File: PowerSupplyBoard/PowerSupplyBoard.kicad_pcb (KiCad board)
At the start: 4 copper layers, 50 x 75 mm, 80 parts, among them J101 BATTERY, J102 DATA2, J103 USB_C, J104 PWR, J105 DATA1, J106 USB_B_Micro, Q101 BSH205G2A, Q102 TD6790, Q103 TD6790, Q104 TD6790, SW101 SW_SPDT, U101 TPS63021, U102 MCP73834T, U103 TC7662Bx0A, U104 TC7662Bx0A, U105 CS5173

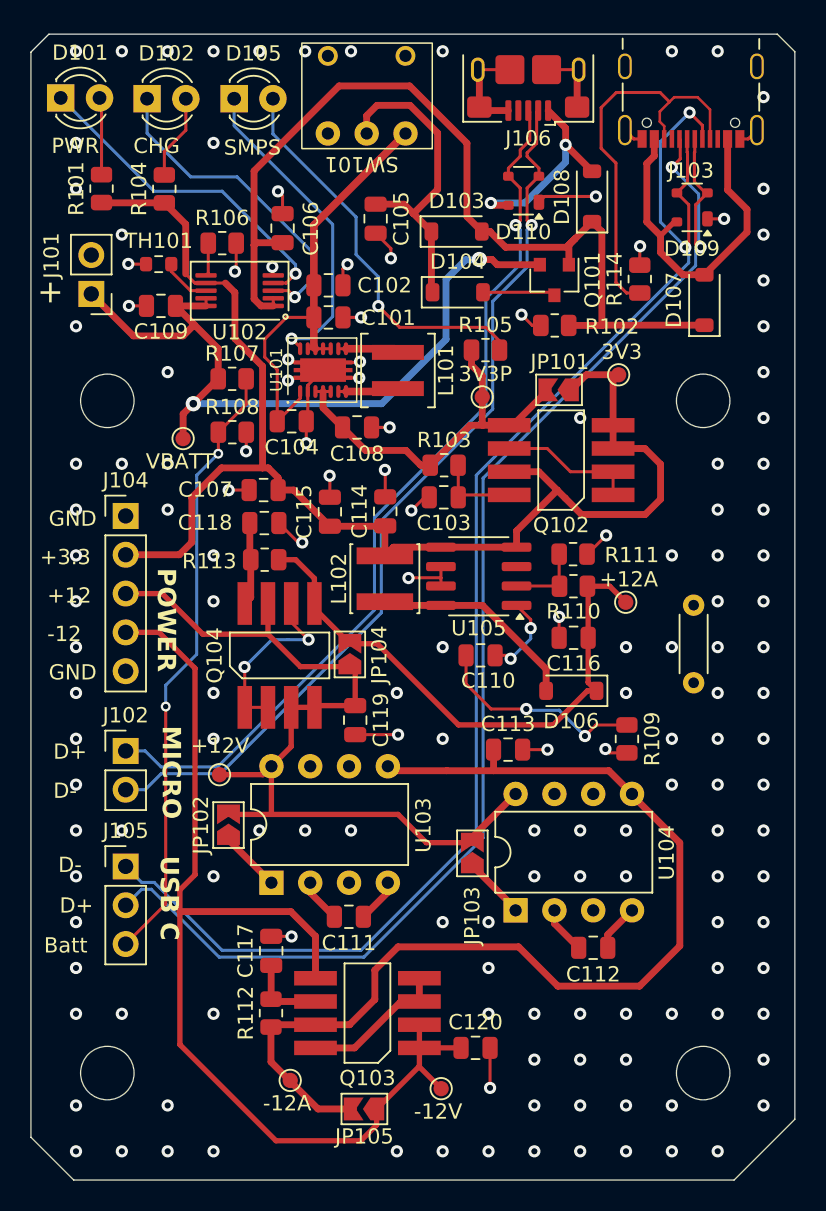
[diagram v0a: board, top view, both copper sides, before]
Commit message: Power board rev 3
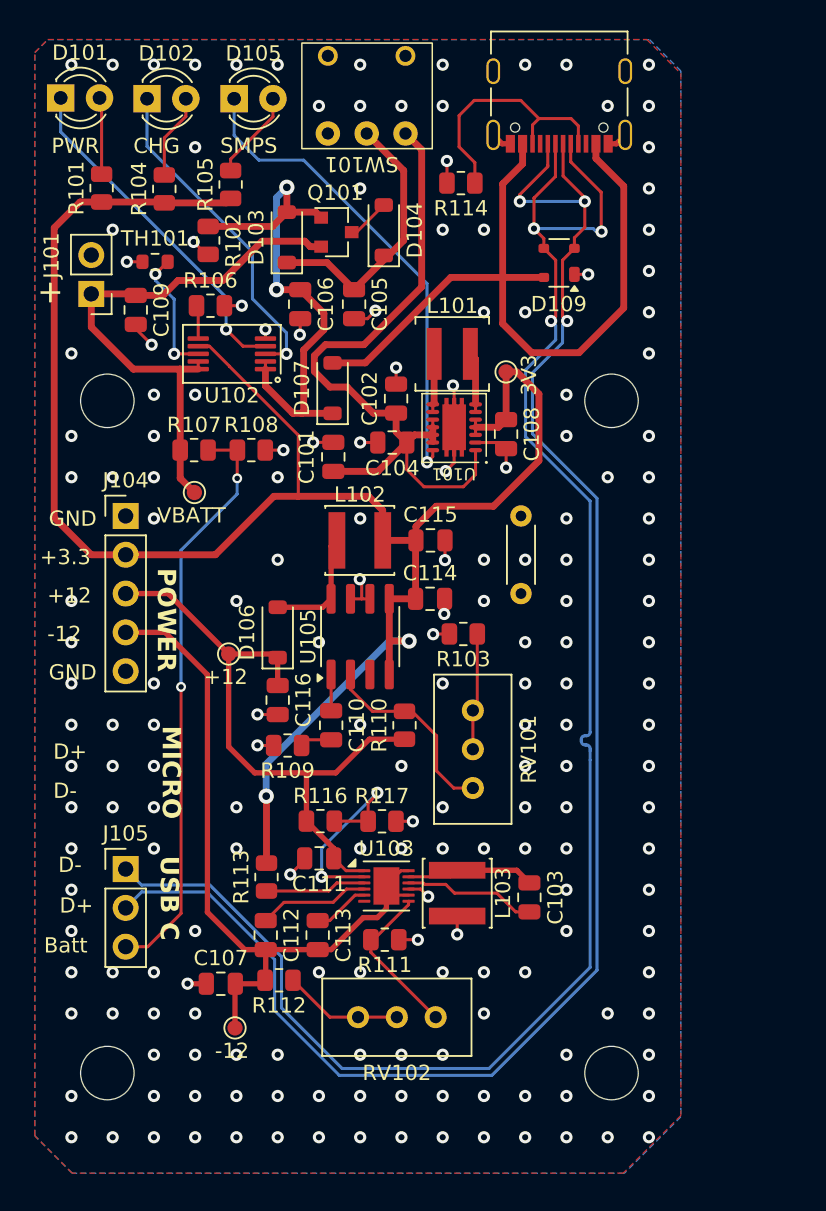
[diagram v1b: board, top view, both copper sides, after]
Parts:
- removed C117, C118: 1u, Capacitor_SMD:C_0805_2012Metric
- removed C119, C120: 100n, Capacitor_SMD:C_0805_2012Metric
- removed D108: PMEG3030, Diode_SMD:D_SOD-123
- removed D110: SP0503BAHT, Package_TO_SOT_SMD:SOT-143
- removed J102: DATA2, Connector_PinHeader_2.54mm:PinHeader_1x02_P2.54mm_Vertical
- removed J106: USB_B_Micro, Connector_USB:USB_Micro-B_Amphenol_10118193-0001LF_Horizontal
- removed JP101: DIG_CM, Jumper:SolderJumper-2_Open_TrianglePad_0805
- removed JP102, JP103: INV_HIFREQ, Jumper:SolderJumper-2_Open_TrianglePad_0805
- removed JP104: POS_CM, Jumper:SolderJumper-2_Open_TrianglePad_0805
- removed JP105: NEG_CM, Jumper:SolderJumper-2_Open_TrianglePad_0805
- removed Q102, Q103, Q104: TD6790, PCM_4ms_Package_SOIC:SM-8
- removed TP104: -12A, TestPoint:TestPoint_Pad_D1.0mm_Value
- removed TP106: -12V, TestPoint:TestPoint_Pad_D1.0mm_Value
- removed TP107: +12V, TestPoint:TestPoint_Pad_D1.0mm_Value
- removed U104: TC7662Bx0A, Package_DIP:DIP-8_W7.62mm
- added L103: 22uH, Inductor_SMD:L_Changjiang_FNR4010S, F.Cu at (27.9, 56.2)
- added R116: 330k, Resistor_SMD:R_0805_2012Metric, F.Cu at (18.9, 51.5)
- added R117: 100k, Resistor_SMD:R_0805_2012Metric, F.Cu at (23.0, 51.5)
- added RV101: 10k, Potentiometer_THT:Potentiometer_Bourns_3296W_Vertical, F.Cu at (28.9, 49.3)
- added RV102: 10k, Potentiometer_THT:Potentiometer_Bourns_3296W_Vertical, F.Cu at (26.5, 64.3)
- C103: value 22u -> 100n
- C107: value 100n -> 22u
- C111: value 10u -> 4u7
- C112: value 10u -> 4n7
- C113: value 10u -> 2u2
- R103: value 10k -> 1k
- R111: value 4k7 -> 470k
- R112: value 12k -> 33k
- R113: value 12k -> 4k7
- TP101: value 3V3 -> -12
- TP102: value 3V3P -> 3V3
- TP105: value +12A -> +12
- U103: value TC7662Bx0A -> MAX17578ATC; footprint Package_DIP:DIP-8_W7.62mm -> Package_DFN_QFN:TDFN-12-1EP_3x3mm_P0.4mm_EP1.7x2.45mm
- moved TP101 49.6 mm to (13.4, 65.0), turned to 180 degrees
- moved C107 32.4 mm to (12.4, 62.2), turned to 0 degrees
- moved R111 28.1 mm to (23.2, 59.3), turned to 180 degrees
- moved C103 26.8 mm to (32.6, 56.5), turned to 90 degrees
- moved TP105 26.2 mm to (12.9, 40.6), turned to 180 degrees
- moved D107 25.0 mm to (19.7, 23.2)
- moved R102 23.4 mm to (11.6, 13.5), turned to -90 degrees
- moved R109 22.2 mm to (16.8, 46.6), turned to 180 degrees
- moved C112 21.5 mm to (15.4, 59.0), turned to -90 degrees
- moved R113 20.8 mm to (15.4, 55.2), turned to 90 degrees
- moved R105 19.9 mm to (13.1, 9.84), turned to 90 degrees
- moved C116 19.8 mm to (16.1, 43.6), turned to -90 degrees
- moved D106 19.6 mm to (16.1, 39.2), turned to 90 degrees
- moved C113 17.4 mm to (18.8, 59.0), turned to -90 degrees
- moved Q101 14.6 mm to (20.0, 13.0), turned to 0 degrees
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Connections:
- C103 pad 1: Net-(Q102A-B1) -> Net-(U103-BST)
- C103 pad 2: GND -> Net-(U103-LX)
- C107 pad 1: +3.3V -> GND
- C107 pad 2: GND -> -12V
- C108 pad 1: +3.3VP -> +3.3V
- C111 pad 1: Net-(U103-CAP+) -> +12V
- C111 pad 2: Net-(U103-CAP-) -> GND
- C112 pad 1: Net-(U104-CAP+) -> Net-(U103-SS)
- C112 pad 2: Net-(U104-CAP-) -> -12V
- C113 pad 1: -12VA -> Net-(U103-VCC)
- C113 pad 2: GND -> -12V
- C116 pad 1: +12VA -> +12V
- D106 pad 1: +12VA -> +12V
- R103 pad 1: +3.3VP -> Net-(R103-Pad1)
- R103 pad 2: Net-(Q102A-B1) -> GND
- R105 pad 1: +3.3VP -> +3.3V
- R110 pad 1: +12VA -> +12V
- R111 pad 1: Net-(U105-FB) -> GND
- R111 pad 2: GND -> Net-(U103-FB)
- R112 pad 1: -12VA -> Net-(R112-Pad1)
- R112 pad 2: Net-(Q103B-B2) -> -12V
- R113 pad 1: +12VA -> /NRST
- R113 pad 2: Net-(Q104A-B1) -> +3.3V
- TP101 pad 1: +3.3V -> -12V
- TP102 pad 1: +3.3VP -> +3.3V
- TP105 pad 1: +12VA -> +12V
- U101 pad 3: +3.3VP -> +3.3V
- U101 pad 4: +3.3VP -> +3.3V
- U101 pad 5: +3.3VP -> +3.3V
- U103 pad 1: Net-(JP102-A) -> +12V
- U103 pad 2: Net-(U103-CAP+) -> Net-(U103-EN/UVLO)
- U103 pad 3: GND -> /NRST
- U103 pad 4: Net-(U103-CAP-) -> Net-(U103-SS)
- U103 pad 5: -12VA -> Net-(U103-VCC)
- U103 pad 7: unconnected-(U103-OSC-Pad7) -> Net-(U103-FB)
- U103 pad 8: +12V -> -12V
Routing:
- net -12VA: track 70.5 -> 0.00 mm
- net USBM_D-: track 59.5 -> 0.00 mm, vias 1 -> 0
- net USBM_D+: track 58.8 -> 0.00 mm, vias 1 -> 0
- net +3.3V: track 89.8 -> 128.1 mm, vias 0 -> 2
- net +12VA: track 37.4 -> 0.00 mm
- net VDD: track 62.4 -> 34.2 mm, vias 0 -> 2
- net GND: track 68.5 -> 40.7 mm, vias 155 -> 189
- net Net-(D107-A): track 23.5 -> 49.9 mm
- net +3.3VP: track 25.6 -> 0.00 mm
- net -12V: track 71.3 -> 47.9 mm
- net Net-(D105-A): track 25.9 -> 5.85 mm, vias 1 -> 0
- net USBC_D+: track 89.5 -> 108.0 mm, vias 2 -> 3
- net USBC_D-: track 92.9 -> 110.2 mm, vias 2 -> 3
- net V_PWR: track 30.2 -> 46.7 mm
- net +12V: track 57.9 -> 41.4 mm
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- added copper zone on B.Cu, net GND
- added copper zone on F.Cu, net GND
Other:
- board outline removed
- board text removed: "Rev. 2 July 2024 Hayden Setlik"
- board text removed: "USB Synth Power Supply"
